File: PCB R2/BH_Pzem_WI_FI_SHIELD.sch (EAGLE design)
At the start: 27 parts, among them J6 8p, J7 8p, U2 esp12

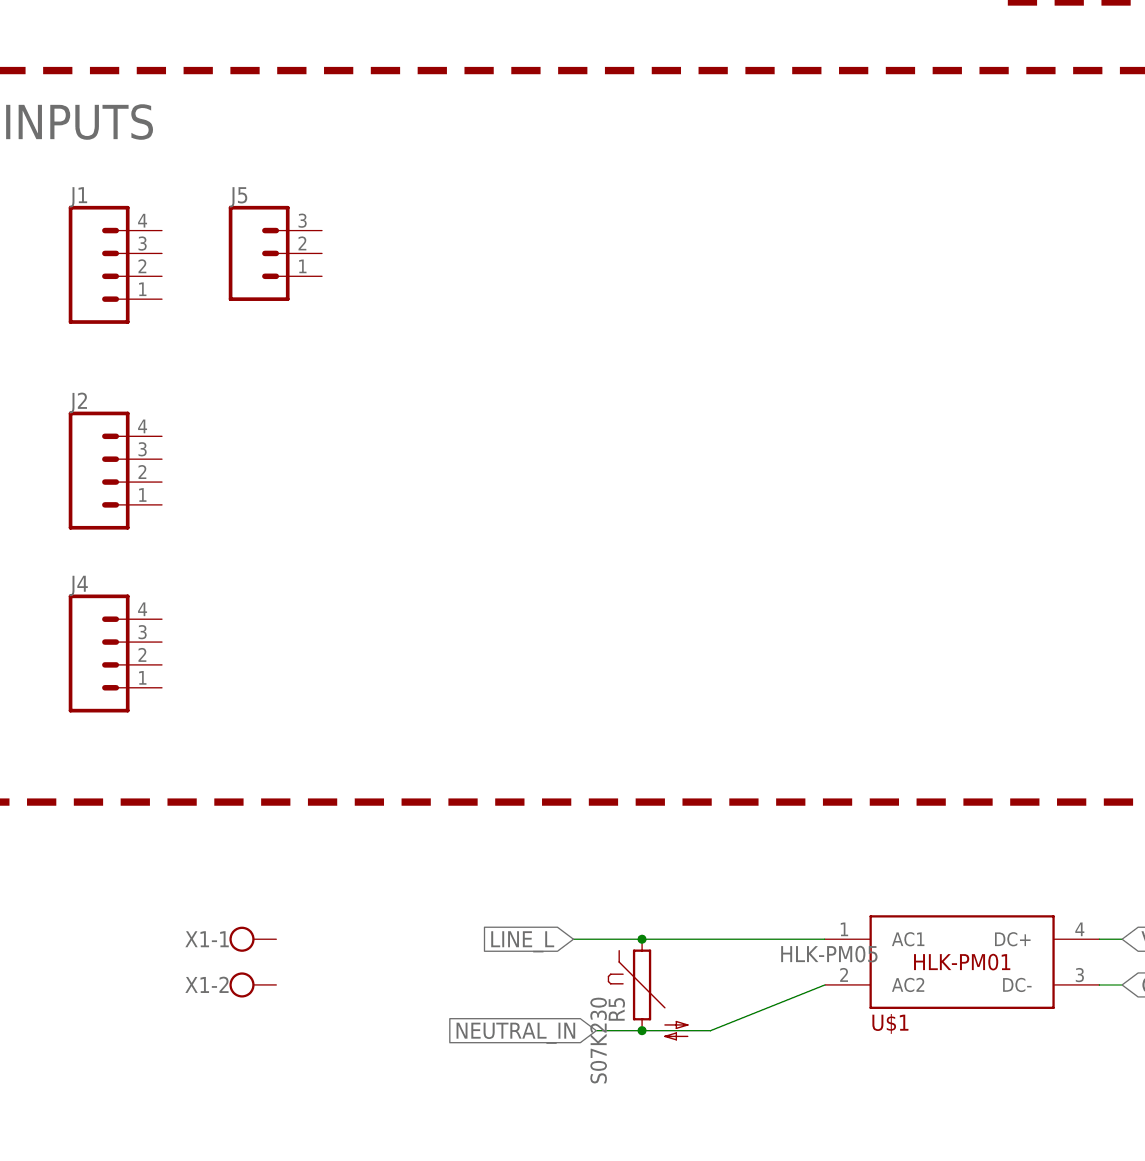
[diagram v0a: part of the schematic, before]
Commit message: rev2
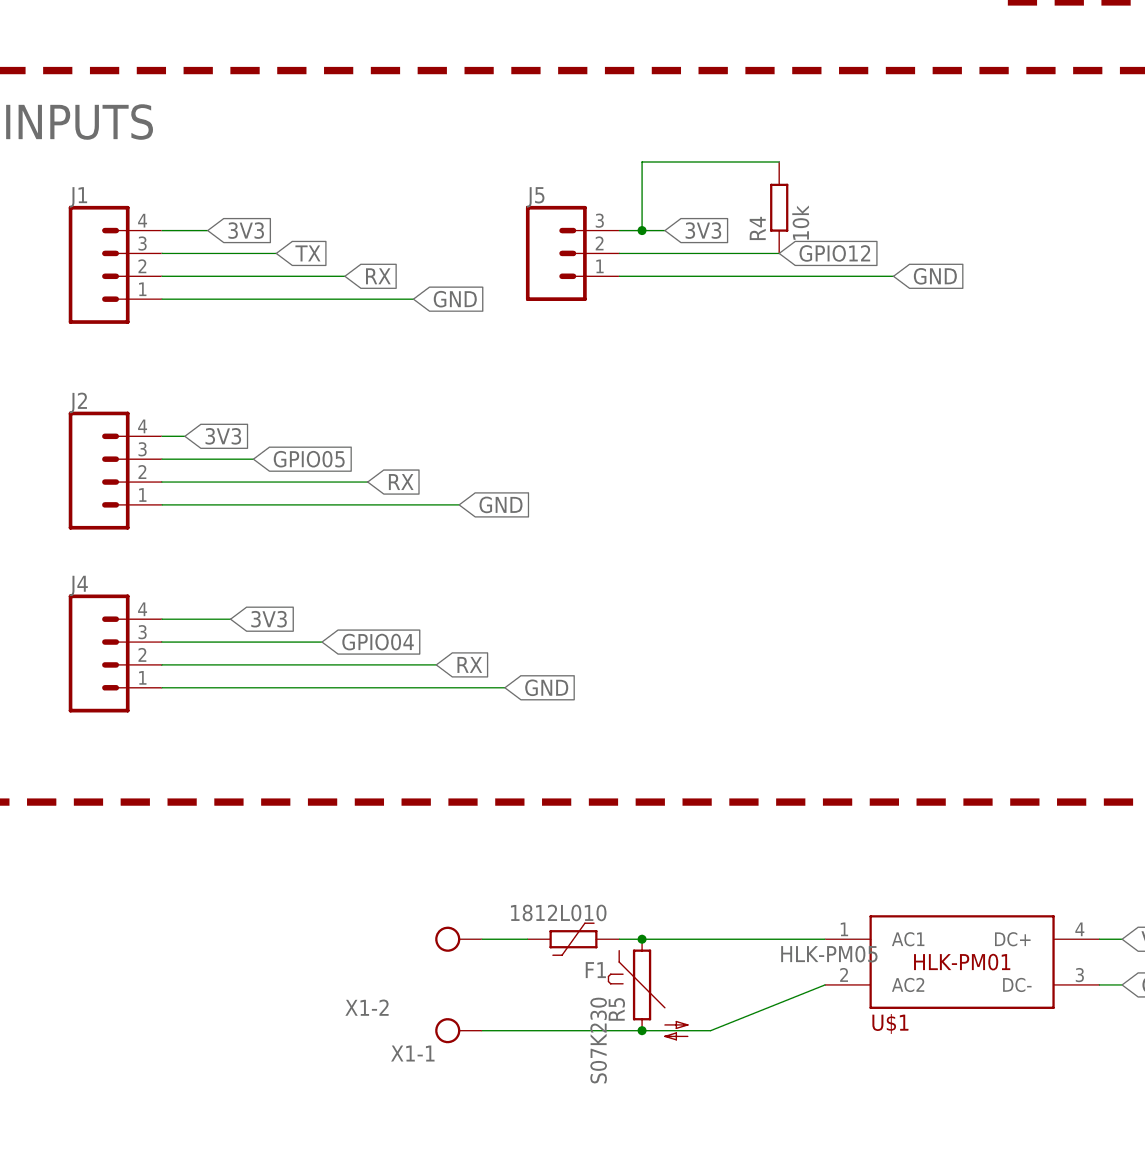
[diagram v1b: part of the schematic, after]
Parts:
- added F1: 1812L010, polyfuse-smd_10:1812L010
- added R4: 10k, resistor:R-EU_R0603
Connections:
- new net N$2: F1.1, X1-2.KL
- net 3V3: now also J1.4, J2.4, J4.4, J5.3, R4.2
- net GND: now also J1.1, J2.1, J4.1, J5.1
- net GPIO04: now also J4.3
- net GPIO05: now also J2.3
- net GPIO12: now also J5.2, R4.1
- net LINE_L: now also F1.2
- net NEUTRAL_IN: now also X1-1.KL
- net RX: now also J1.2, J2.2, J4.2
- net TX: now also J1.3
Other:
- moved on the sheet: J5, X1-1, X1-2
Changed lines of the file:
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@@
 <part name="J5" library="SparkFun-Connectors" library_urn="urn:adsk.eagle:library:513" deviceset="CONN_03" device="JST-PTH-VERT" package3d_urn="urn:adsk.eagle:package:38080/1"/>
 <part name="X1" library="con-wago-500" library_urn="urn:adsk.eagle:library:195" deviceset="W237-102" device="" package3d_urn="urn:adsk.eagle:package:10688/1"/>
+<part name="F1" library="polyfuse-smd_10" deviceset="?" device="1812L" technology="010"/>
+<part name="R4" library="resistor" library_urn="urn:adsk.eagle:library:348" deviceset="R-EU_" device="R0603" package3d_urn="urn:adsk.eagle:package:26057/1" value="10k"/>
 </parts>
 <sheets>
@@
 <attribute name="VALUE" x="5.842" y="59.69" size="1.778" layer="96" rot="R90"/>
 </instance>
-<instance part="J5" gate="J$1" x="68.58" y="93.98" smashed="yes">
-<attribute name="VALUE" x="66.04" y="86.614" size="1.778" layer="96" font="vector"/>
-<attribute name="NAME" x="66.04" y="99.568" size="1.778" layer="95" font="vector"/>
-</instance>
-<instance part="X1" gate="-1" x="66.04" y="17.78" smashed="yes">
-<attribute name="NAME" x="66.04" y="18.669" size="1.778" layer="95" rot="R180"/>
-</instance>
-<instance part="X1" gate="-2" x="66.04" y="12.7" smashed="yes">
-<attribute name="VALUE" x="63.5" y="9.017" size="1.778" layer="96"/>
-<attribute name="NAME" x="66.04" y="13.589" size="1.778" layer="95" rot="R180"/>
+<instance part="J5" gate="J$1" x="101.6" y="93.98" smashed="yes">
+<attribute name="VALUE" x="99.06" y="86.614" size="1.778" layer="96" font="vector"/>
+<attribute name="NAME" x="99.06" y="99.568" size="1.778" layer="95" font="vector"/>
+</instance>
+<instance part="X1" gate="-1" x="88.9" y="7.62" smashed="yes">
+<attribute name="NAME" x="88.9" y="5.969" size="1.778" layer="95" rot="R180"/>
+</instance>
+<instance part="X1" gate="-2" x="88.9" y="17.78" smashed="yes">
+<attribute name="VALUE" x="86.36" y="14.097" size="1.778" layer="96"/>
+<attribute name="NAME" x="83.82" y="11.049" size="1.778" layer="95" rot="R180"/>
+</instance>
+<instance part="F1" gate="G$1" x="104.14" y="17.78" smashed="yes" rot="R180">
+<attribute name="NAME" x="107.95" y="15.24" size="1.778" layer="95" rot="R180"/>
+<attribute name="VALUE" x="107.95" y="21.59" size="1.778" layer="96" rot="R180"/>
+</instance>
+<instance part="R4" gate="G$1" x="127" y="99.06" smashed="yes" rot="R90">
+<attribute name="NAME" x="125.5014" y="95.25" size="1.778" layer="95" rot="R90"/>
+<attribute name="VALUE" x="130.302" y="95.25" size="1.778" layer="96" rot="R90"/>
 </instance>
 </instances>
@@
 <label x="2.54" y="55.88" size="1.778" layer="95" rot="R270" xref="yes"/>
 </segment>
+<segment>
+<pinref part="J1" gate="G$1" pin="1"/>
+<wire x1="58.42" y1="88.9" x2="86.36" y2="88.9" width="0.1524" layer="91"/>
+<label x="86.36" y="88.9" size="1.778" layer="95" xref="yes"/>
+</segment>
+<segment>
+<pinref part="J2" gate="G$1" pin="1"/>
+<wire x1="58.42" y1="66.04" x2="91.44" y2="66.04" width="0.1524" layer="91"/>
+<label x="91.44" y="66.04" size="1.778" layer="95" xref="yes"/>
+</segment>
+<segment>
+<pinref part="J4" gate="G$1" pin="1"/>
+<wire x1="58.42" y1="45.72" x2="96.52" y2="45.72" width="0.1524" layer="91"/>
+<label x="96.52" y="45.72" size="1.778" layer="95" xref="yes"/>
+</segment>
+<segment>
+<pinref part="J5" gate="J$1" pin="1"/>
+<wire x1="109.22" y1="91.44" x2="139.7" y2="91.44" width="0.1524" layer="91"/>
+<label x="139.7" y="91.44" size="1.778" layer="95" xref="yes"/>
+</segment>
 </net>
 <net name="VCC" class="0">
@@
 <label x="231.14" y="96.52" size="1.778" layer="95" xref="yes"/>
 </segment>
+<segment>
+<pinref part="J1" gate="G$1" pin="2"/>
+<wire x1="58.42" y1="91.44" x2="78.74" y2="91.44" width="0.1524" layer="91"/>
+<label x="78.74" y="91.44" size="1.778" layer="95" xref="yes"/>
+</segment>
+<segment>
+<pinref part="J2" gate="G$1" pin="2"/>
+<wire x1="58.42" y1="68.58" x2="81.28" y2="68.58" width="0.1524" layer="91"/>
+<label x="81.28" y="68.58" size="1.778" layer="95" xref="yes"/>
+</segment>
+<segment>
+<pinref part="J4" gate="G$1" pin="2"/>
+<wire x1="58.42" y1="48.26" x2="88.9" y2="48.26" width="0.1524" layer="91"/>
+<label x="88.9" y="48.26" size="1.778" layer="95" xref="yes"/>
+</segment>
 </net>
 <net name="GPIO04" class="0">
@@
 <label x="231.14" y="91.44" size="1.778" layer="95" xref="yes"/>
 </segment>
+<segment>
+<pinref part="J4" gate="G$1" pin="3"/>
+<wire x1="58.42" y1="50.8" x2="76.2" y2="50.8" width="0.1524" layer="91"/>
+<label x="76.2" y="50.8" size="1.778" layer="95" xref="yes"/>
+</segment>
 </net>
 <net name="GPIO05" class="0">
@@
 <label x="218.44" y="93.98" size="1.778" layer="95" xref="yes"/>
 </segment>
+<segment>
+<pinref part="J2" gate="G$1" pin="3"/>
+<wire x1="58.42" y1="71.12" x2="68.58" y2="71.12" width="0.1524" layer="91"/>
+<label x="68.58" y="71.12" size="1.778" layer="95" xref="yes"/>
+</segment>
 </net>
 <net name="GPIO02" class="0">
@@
 <wire x1="210.82" y1="58.42" x2="226.06" y2="58.42" width="0.1524" layer="91"/>
 <label x="226.06" y="58.42" size="1.778" layer="95" xref="yes"/>
+</segment>
+<segment>
+<pinref part="J5" gate="J$1" pin="2"/>
+<wire x1="109.22" y1="93.98" x2="127" y2="93.98" width="0.1524" layer="91"/>
+<label x="127" y="93.98" size="1.778" layer="95" xref="yes"/>
+<pinref part="R4" gate="G$1" pin="1"/>
 </segment>
 </net>
@@
 <wire x1="-17.78" y1="142.24" x2="-15.24" y2="142.24" width="0.1524" layer="91"/>
 <label x="-15.24" y="142.24" size="1.778" layer="95" xref="yes"/>
+</segment>
+<segment>
+<pinref part="J1" gate="G$1" pin="3"/>
+<wire x1="58.42" y1="93.98" x2="71.12" y2="93.98" width="0.1524" layer="91"/>
+<label x="71.12" y="93.98" size="1.778" layer="95" xref="yes"/>
 </segment>
 </net>
@@
 <junction x="220.98" y="17.78"/>
 </segment>
+<segment>
+<pinref part="J1" gate="G$1" pin="4"/>
+<wire x1="58.42" y1="96.52" x2="63.5" y2="96.52" width="0.1524" layer="91"/>
+<label x="63.5" y="96.52" size="1.778" layer="95" xref="yes"/>
+</segment>
+<segment>
+<pinref part="J2" gate="G$1" pin="4"/>
+<wire x1="58.42" y1="73.66" x2="60.96" y2="73.66" width="0.1524" layer="91"/>
+<label x="60.96" y="73.66" size="1.778" layer="95" xref="yes"/>
+</segment>
+<segment>
+<pinref part="J4" gate="G$1" pin="4"/>
+<wire x1="58.42" y1="53.34" x2="66.04" y2="53.34" width="0.1524" layer="91"/>
+<label x="66.04" y="53.34" size="1.778" layer="95" xref="yes"/>
+</segment>
+<segment>
+<pinref part="J5" gate="J$1" pin="3"/>
+<wire x1="109.22" y1="96.52" x2="111.76" y2="96.52" width="0.1524" layer="91"/>
+<label x="114.3" y="96.52" size="1.778" layer="95" xref="yes"/>
+<pinref part="R4" gate="G$1" pin="2"/>
+<wire x1="111.76" y1="96.52" x2="114.3" y2="96.52" width="0.1524" layer="91"/>
+<wire x1="111.76" y1="96.52" x2="111.76" y2="104.14" width="0.1524" layer="91"/>
+<wire x1="111.76" y1="104.14" x2="127" y2="104.14" width="0.1524" layer="91"/>
+<junction x="111.76" y="96.52"/>
+</segment>
 </net>
 <net name="N$1" class="0">
@@
 <wire x1="132.08" y1="12.7" x2="119.38" y2="7.62" width="0.1524" layer="91"/>
 <wire x1="119.38" y1="7.62" x2="111.76" y2="7.62" width="0.1524" layer="91"/>
-<label x="106.68" y="7.62" size="1.778" layer="95" rot="R180" xref="yes"/>
 <pinref part="U$1" gate="G$1" pin="AC2"/>
 <pinref part="R5" gate="G$1" pin="2"/>
-<wire x1="111.76" y1="7.62" x2="106.68" y2="7.62" width="0.1524" layer="91"/>
+<pinref part="X1" gate="-1" pin="KL"/>
+<wire x1="93.98" y1="7.62" x2="111.76" y2="7.62" width="0.1524" layer="91"/>
 <junction x="111.76" y="7.62"/>
 </segment>
@@
 <segment>
 <wire x1="132.08" y1="17.78" x2="111.76" y2="17.78" width="0.1524" layer="91"/>
-<label x="104.14" y="17.78" size="1.778" layer="95" rot="R180" xref="yes"/>
 <pinref part="U$1" gate="G$1" pin="AC1"/>
 <pinref part="R5" gate="G$1" pin="1"/>
-<wire x1="111.76" y1="17.78" x2="104.14" y2="17.78" width="0.1524" layer="91"/>
 <junction x="111.76" y="17.78"/>
+<wire x1="111.76" y1="17.78" x2="109.22" y2="17.78" width="0.1524" layer="91"/>
+<pinref part="F1" gate="G$1" pin="2"/>
 </segment>
 </net>
@@
 </segment>
 </net>
+<net name="N$2" class="0">
+<segment>
+<pinref part="X1" gate="-2" pin="KL"/>
+<pinref part="F1" gate="G$1" pin="1"/>
+<wire x1="93.98" y1="17.78" x2="99.06" y2="17.78" width="0.1524" layer="91"/>
+</segment>
+</net>

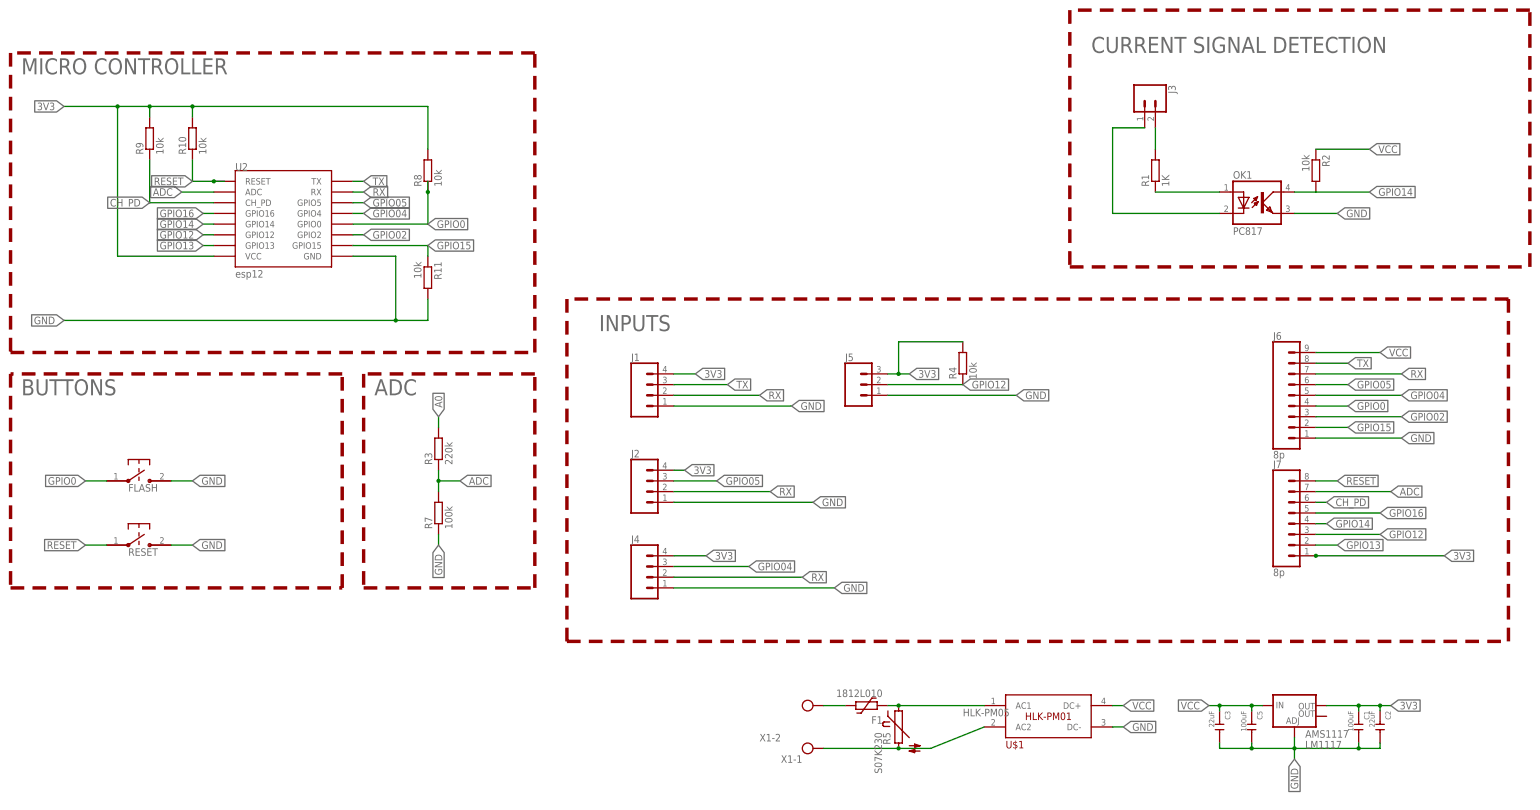
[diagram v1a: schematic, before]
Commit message: v2
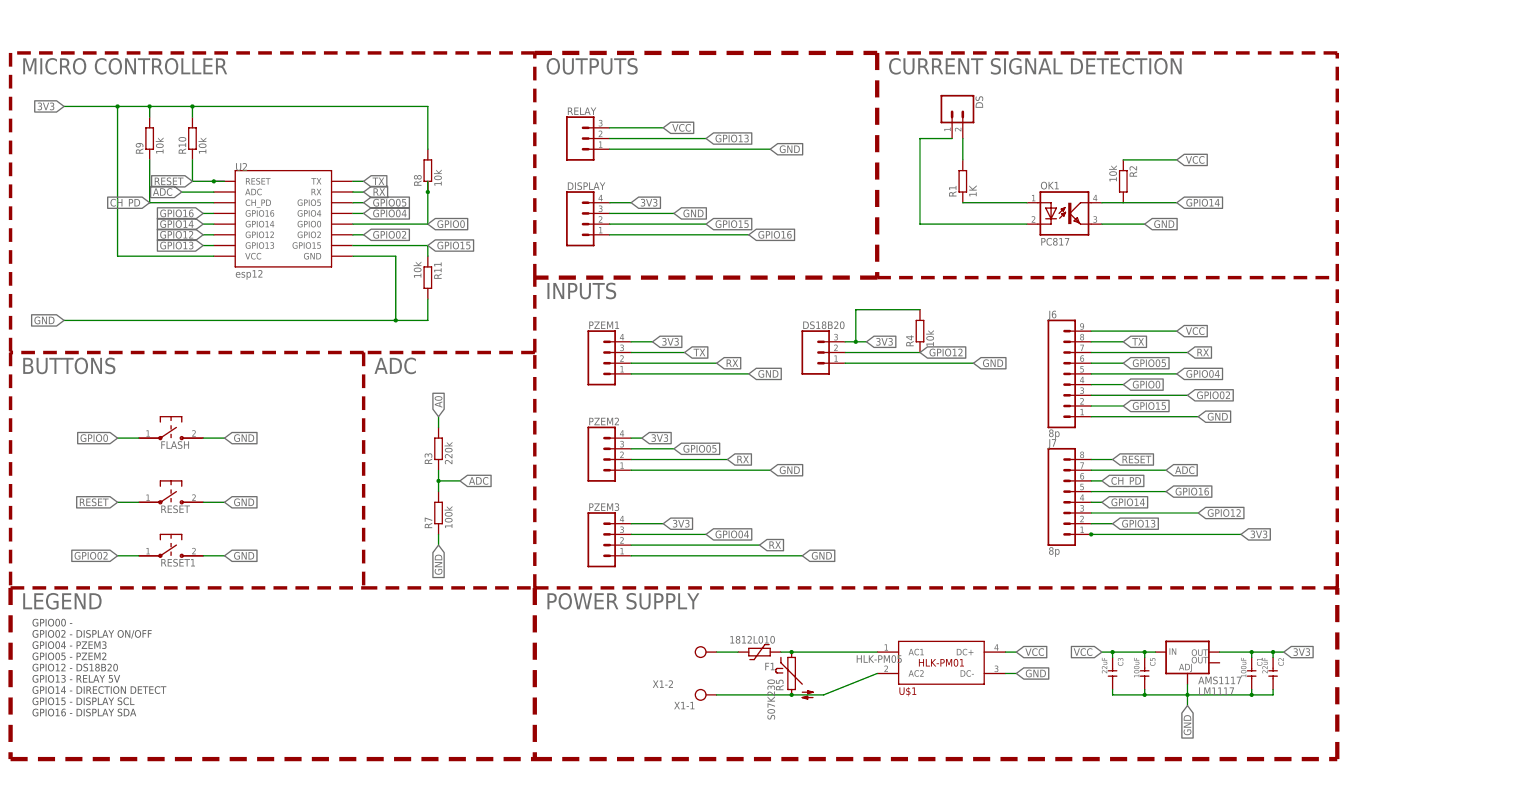
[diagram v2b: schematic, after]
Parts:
- removed J1, J2, J4: (no value), SparkFun-Connectors:CONN_04JST-PTH-VERT
- removed J3: (no value), SparkFun-Connectors:CONN_02
- removed J5: (no value), SparkFun-Connectors:CONN_03JST-PTH-VERT
- added DISPLAY, PZEM1, PZEM2, PZEM3: (no value), SparkFun-Connectors:CONN_04JST-PTH-VERT
- added DS: (no value), SparkFun-Connectors:CONN_02
- added DS18B20, RELAY: (no value), SparkFun-Connectors:CONN_03JST-PTH-VERT
- added RESET1: B3U-1000P-2P-SMD, switches:B3U-1000P
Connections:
- net 3V3: now also DISPLAY.4, DS18B20.3, PZEM1.4, PZEM2.4, PZEM3.4; no longer J1.4, J2.4, J4.4, J5.3
- net GND: now also DISPLAY.3, DS18B20.1, PZEM1.1, PZEM2.1, PZEM3.1, RELAY.1, RESET1.P$2; no longer J1.1, J2.1, J4.1, J5.1
- net GPIO02: now also RESET1.P$1
- net GPIO04: now also PZEM3.3; no longer J4.3
- net GPIO05: now also PZEM2.3; no longer J2.3
- net GPIO12: now also DS18B20.2; no longer J5.2
- net GPIO13: now also RELAY.2
- net GPIO15: now also DISPLAY.2
- net GPIO16: now also DISPLAY.1
- net N$3: now also DS.2; no longer J3.2
- net RX: now also PZEM1.2, PZEM2.2, PZEM3.2; no longer J1.2, J2.2, J4.2
- net SIGNAL_GND: now also DS.1; no longer J3.1
- net TX: now also PZEM1.3; no longer J1.3
- net VCC: now also RELAY.3
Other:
- note added: "GPIO00 - GPIO02 - DISPLAY ON/OFF GPIO04 - PZEM3 GPIO05 - PZEM2 GPIO12 - DS18B20 GPIO13 - RELAY 5V GPIO14 - DIRECTION DETECT GPIO15 - DISPLAY SCL GPIO16 - DISPLAY SDA"
- note added: "LEGEND"
- note added: "OUTPUTS"
- note added: "POWER SUPPLY"
- moved on the sheet: AMS1117, C1, C2, C3, C5, F1, FLASH, J6, J7, OK1, R1, R2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
